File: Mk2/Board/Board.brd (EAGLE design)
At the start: 47 x 44.1 mm, 7 parts

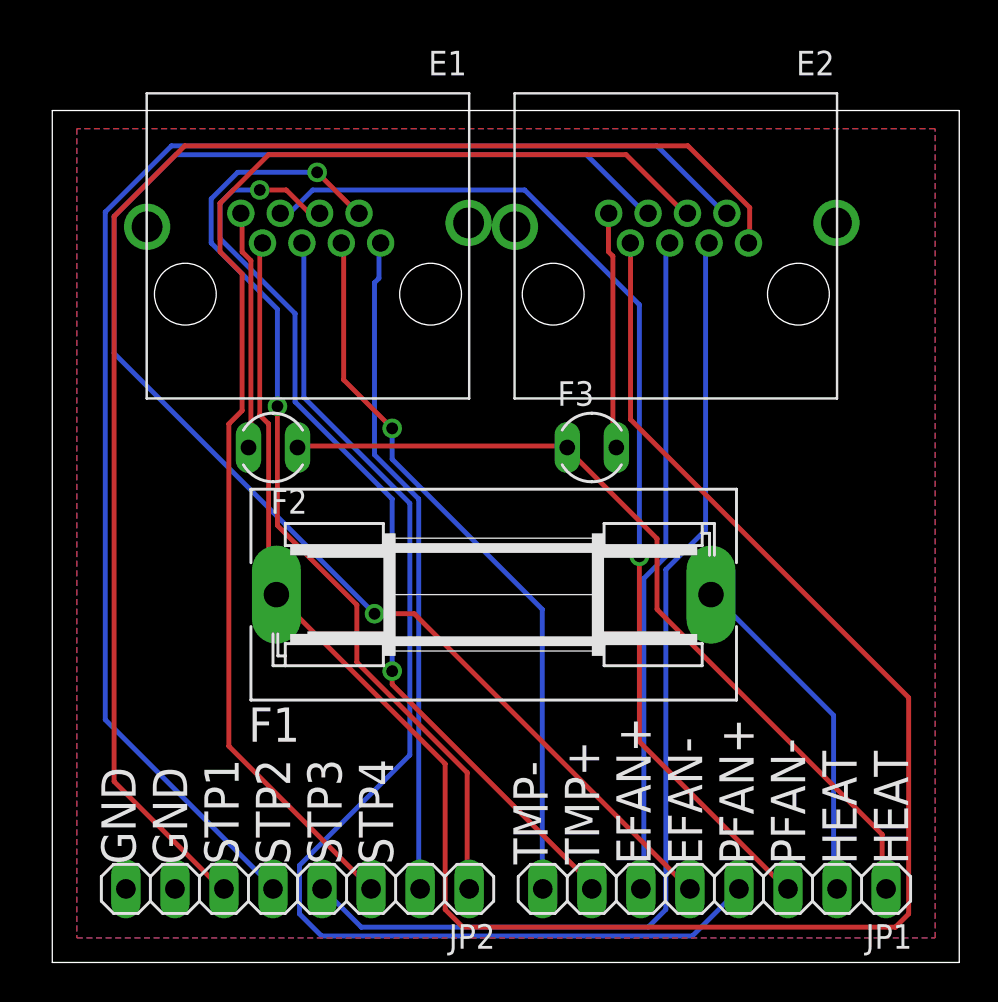
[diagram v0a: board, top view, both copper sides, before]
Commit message: board design
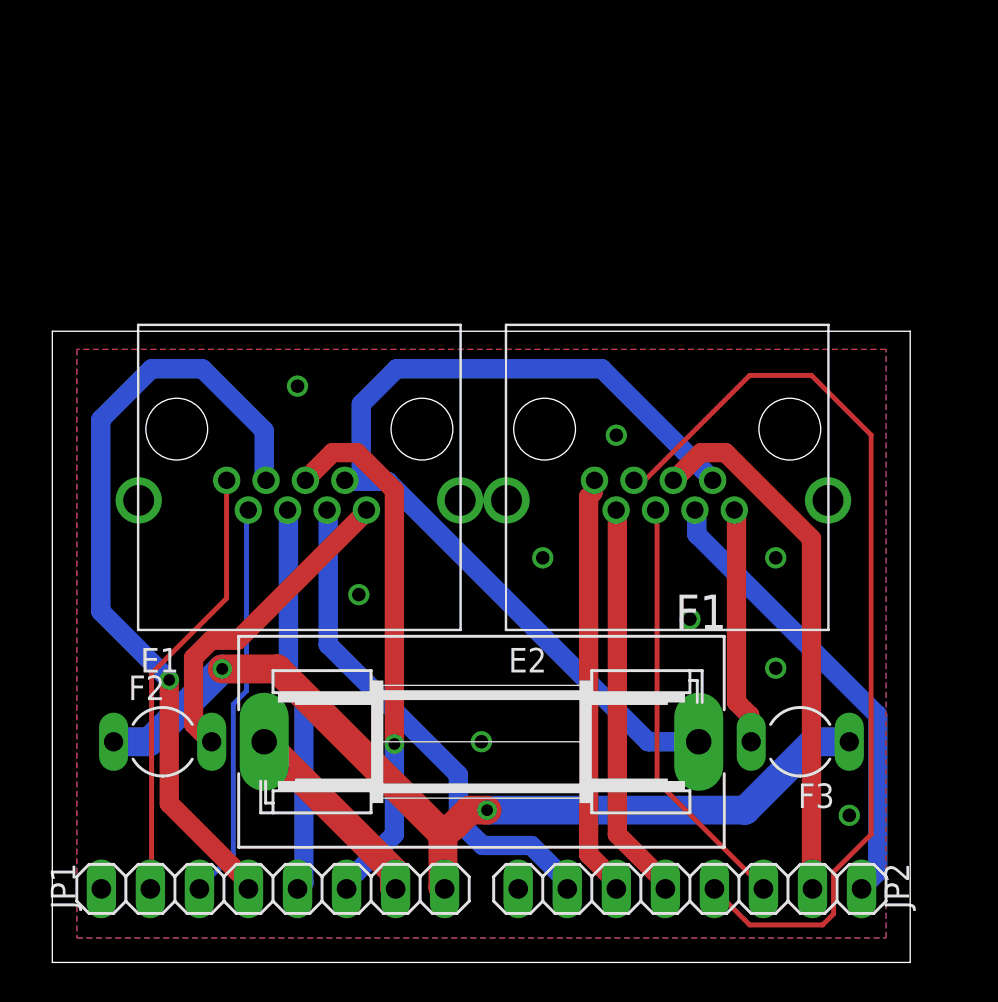
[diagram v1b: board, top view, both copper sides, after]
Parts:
- F2, F3: device ptc-ntc:P679 -> bardiir:POLYFUSE
- moved JP1 22.9 mm to (11.4, 3.81)
- moved JP2 20.3 mm to (33.0, 3.81)
- moved F3 18.7 mm to (38.7, 11.4), turned to 180 degrees
- moved E1 17.6 mm to (4.45, 33.0), turned to 0 degrees
- moved E2 17.6 mm to (23.5, 33.0), turned to 0 degrees
- moved F2 16.3 mm to (5.71, 11.4), turned to 0 degrees
- moved F1 7.65 mm to (22.2, 11.4), turned to 180 degrees
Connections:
- removed net N$12: E1.2, JP2.1
- removed net N$13 (its old number): E1.1, JP2.2
- new net N$17: E2.5, JP2.2
- new net N$18: E2.6, JP2.1
- net GND: now also E1.S@1, E1.S@2, E2.S@1, E2.S@2, JP1.8; no longer E1.S1, E1.S2, E2.S1, E2.S2, JP2.7
- net N$10: now also E1.5, JP1.3; no longer E1.4, JP1.7
- net N$11: now also E1.6, JP2.7; no longer E1.3, JP1.8
- net N$6: now also E1.1, JP1.7; no longer E1.6, JP1.3
- net N$7: now also E1.2, JP1.6; no longer E1.5, JP1.4
- net N$8: now also E1.3; no longer E2.6
- net N$9: now also E1.4, JP1.4; no longer E2.5, JP1.6
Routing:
- net N$3: track 103.9 -> 49.3 mm
- net N$14: track 73.7 -> 20.7 mm
- net N$13: track 74.9 -> 21.9 mm
- net N$12: track 50.4 -> 0.00 mm, vias 2 -> 0
- net N$16: track 65.8 -> 21.9 mm
- net N$7: track 63.7 -> 20.7 mm
- net N$8: track 78.6 -> 41.0 mm
- net N$13 (its old number): track 34.5 -> 0.00 mm
- net N$6: track 55.0 -> 22.8 mm, vias 1 -> 0
- net N$17: track 0.00 -> 27.7 mm
- net N$18: track 0.00 -> 23.9 mm
- net N$10: track 49.6 -> 27.7 mm, vias 2 -> 1
- net N$9: track 34.1 -> 20.1 mm
- net N$11: track 37.7 -> 26.2 mm, vias 1 -> 0
- net N$5: track 18.0 -> 10.4 mm
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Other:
- board size 47 x 44.1 mm -> 44.4 x 32.7 mm
- board text added: "GND EFAN+ EFAN- E1 STP0 STP1 HEAT HEAT GND E2 STP2 STP3 PFAN+ PFAN- TMP+ TMP-"
- board text removed: "GND GND STP1 STP2 STP3 STP4 TMP- TMP+ EFAN+ EFAN- PFAN+ PFAN- HEAT HEAT"
